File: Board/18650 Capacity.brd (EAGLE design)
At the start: 99.1 x 83.7 mm, 58 parts, among them IC1 ATMEGA328-20P

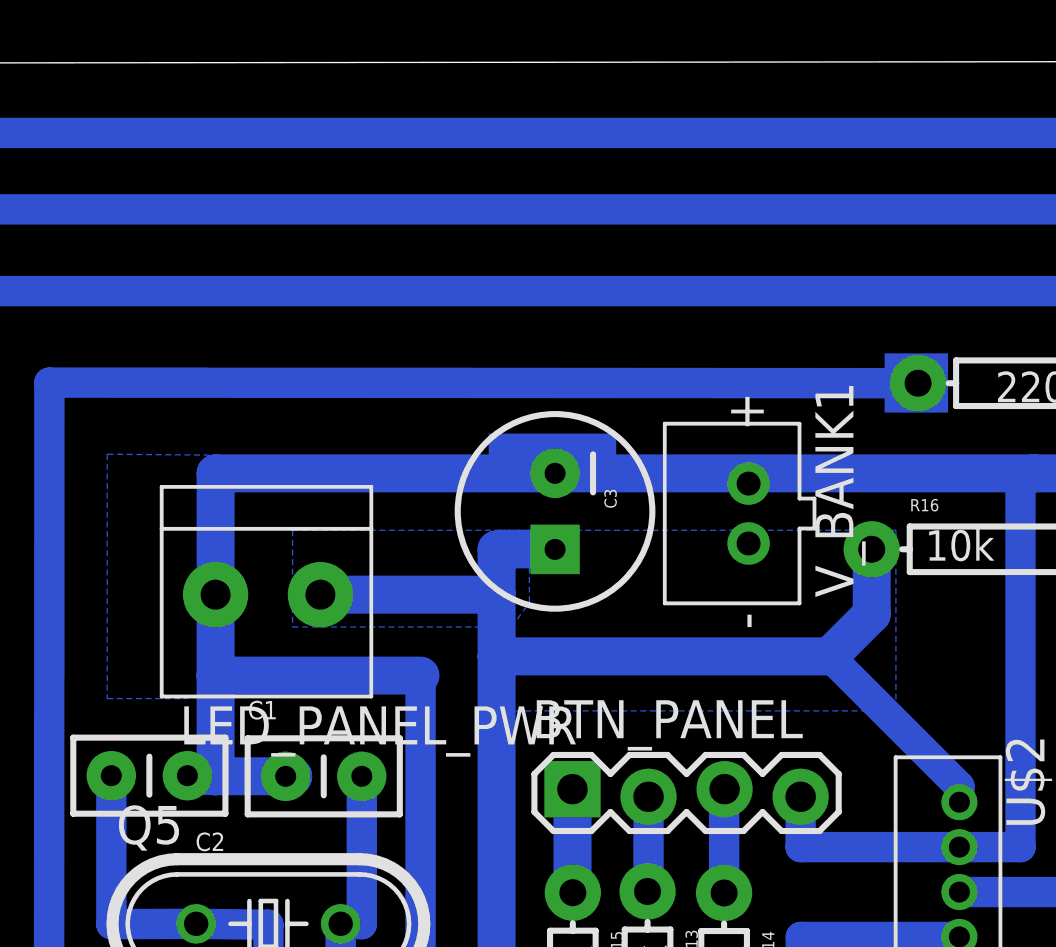
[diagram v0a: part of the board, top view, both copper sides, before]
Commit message: Board Update
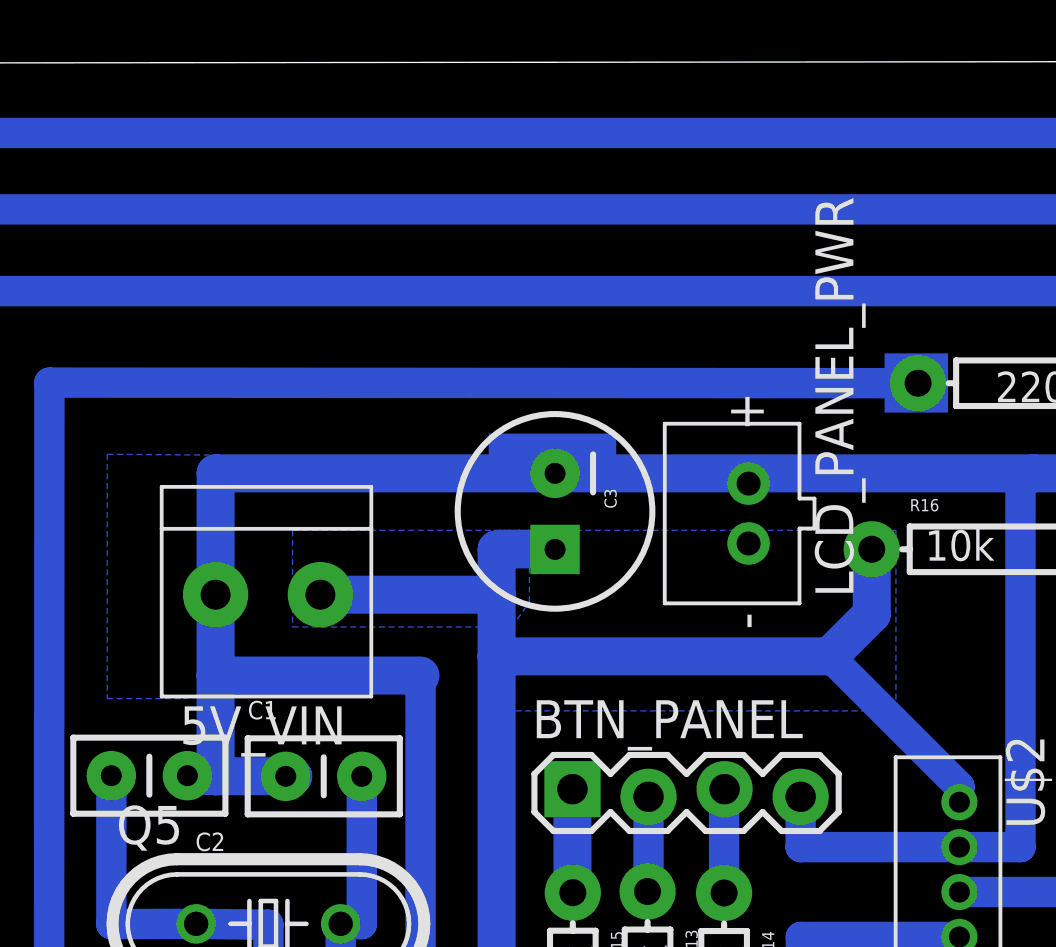
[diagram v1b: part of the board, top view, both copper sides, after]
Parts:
- renumbered LED_PANEL_PWR to 5V_VIN, V_BANK1 to LCD_PANEL_PWR
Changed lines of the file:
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@@
 <element name="C5" library="SparkFun-Passives" package="AXIAL-5MM" value="" x="48.362" y="49.214" rot="R90"/>
 <element name="IC1" library="atmega328" package="DIL28-3" value="ATMEGA328-20P" x="24.054" y="41.326" rot="R180"/>
-<element name="LED_PANEL_PWR" library="adafruit" package="1X2-3.5MM" value="1X2-3.5MM" x="17.74" y="65.81" rot="R180"/>
+<element name="5V_VIN" library="adafruit" package="1X2-3.5MM" value="1X2-3.5MM" x="17.74" y="65.81" rot="R180"/>
 <element name="LED_PANEL" library="SparkFun-Connectors" package="1X04_LOCK" value="" x="10.38" y="51.928" rot="R180"/>
 <element name="JP6" library="SparkFun-Connectors" package="1X02_LOCK" value="" x="28.514" y="20.924" rot="R270"/>
@@
 <element name="FAN_PIN" library="SparkFun-Connectors" package="1X01" value="" x="4.46" y="35.39"/>
 <element name="V_BANK" library="adafruit" package="JST-PH-2-THM" value="" x="19.12" y="20.41" rot="R90"/>
-<element name="V_BANK1" library="adafruit" package="JST-PH-2-THM" value="" x="33.74" y="68.52" rot="R90"/>
+<element name="LCD_PANEL_PWR" library="adafruit" package="JST-PH-2-THM" value="" x="33.74" y="68.52" rot="R90"/>
 </elements>
 <signals>
 <signal name="GND">
 <contactref element="C3" pad="2"/>
-<contactref element="LED_PANEL_PWR" pad="1"/>
+<contactref element="5V_VIN" pad="1"/>
 <contactref element="Q3" pad="3"/>
 <contactref element="Q2" pad="3"/>
@@
 <wire x1="19.12" y1="21.41" x2="19.12" y2="21.98" width="1.016" layer="16"/>
 <wire x1="19.12" y1="21.98" x2="1.55" y2="21.98" width="1.016" layer="16"/>
-<contactref element="V_BANK1" pad="1"/>
+<contactref element="LCD_PANEL_PWR" pad="1"/>
 <wire x1="33.74" y1="69.52" x2="33.398" y2="69.862" width="1.016" layer="16"/>
 <wire x1="33.398" y1="69.862" x2="27.276" y2="69.862" width="1.016" layer="16"/>
@@
 <contactref element="IC1" pad="7"/>
 <contactref element="C3" pad="1"/>
-<contactref element="LED_PANEL_PWR" pad="2"/>
+<contactref element="5V_VIN" pad="2"/>
 <contactref element="L1" pad="1"/>
 <contactref element="R16" pad="P$1"/>
@@
 <wire x1="22.4222" y1="18.49" x2="22.4222" y2="22.36" width="1.016" layer="16"/>
 <wire x1="22.4222" y1="22.36" x2="22.4122" y2="22.36" width="1.016" layer="16"/>
-<contactref element="V_BANK1" pad="2"/>
+<contactref element="LCD_PANEL_PWR" pad="2"/>
 <polygon width="0.254" layer="16" thermals="no">
 <vertex x="21.83" y="18.2"/>
